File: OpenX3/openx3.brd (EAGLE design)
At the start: 46.7 x 49.1 mm, 34 parts, among them IC1 24AA256SN, J1 BM20B-SRDS-G-TF(LF)(SN), J2 SM12B-SRSS-TB(LF)(SN), J3 53398-0271, J4 1734260-3, U1 LC4256V-75TN100CTQFP100-L, U2 AM29F016D-70EF, U3 AM29F002BB90EI

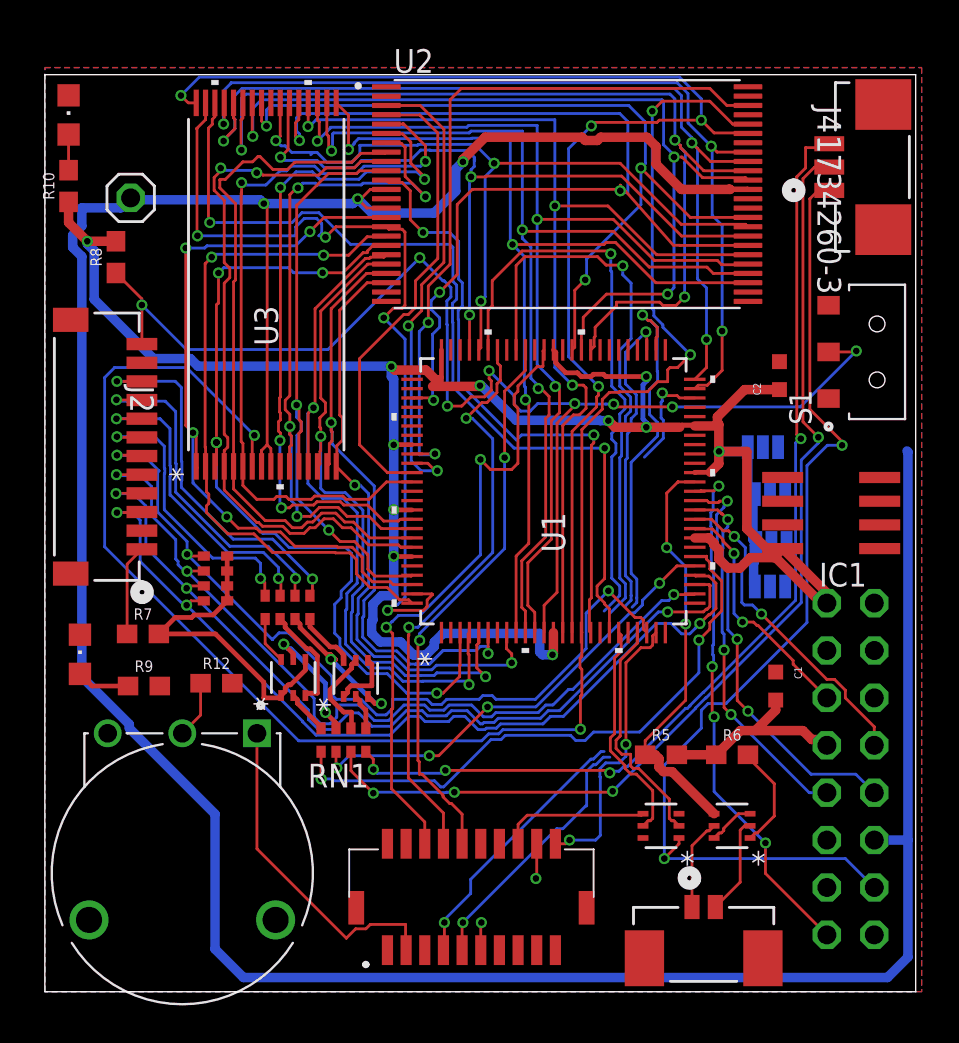
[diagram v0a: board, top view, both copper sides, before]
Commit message: routing complete... passes DRC
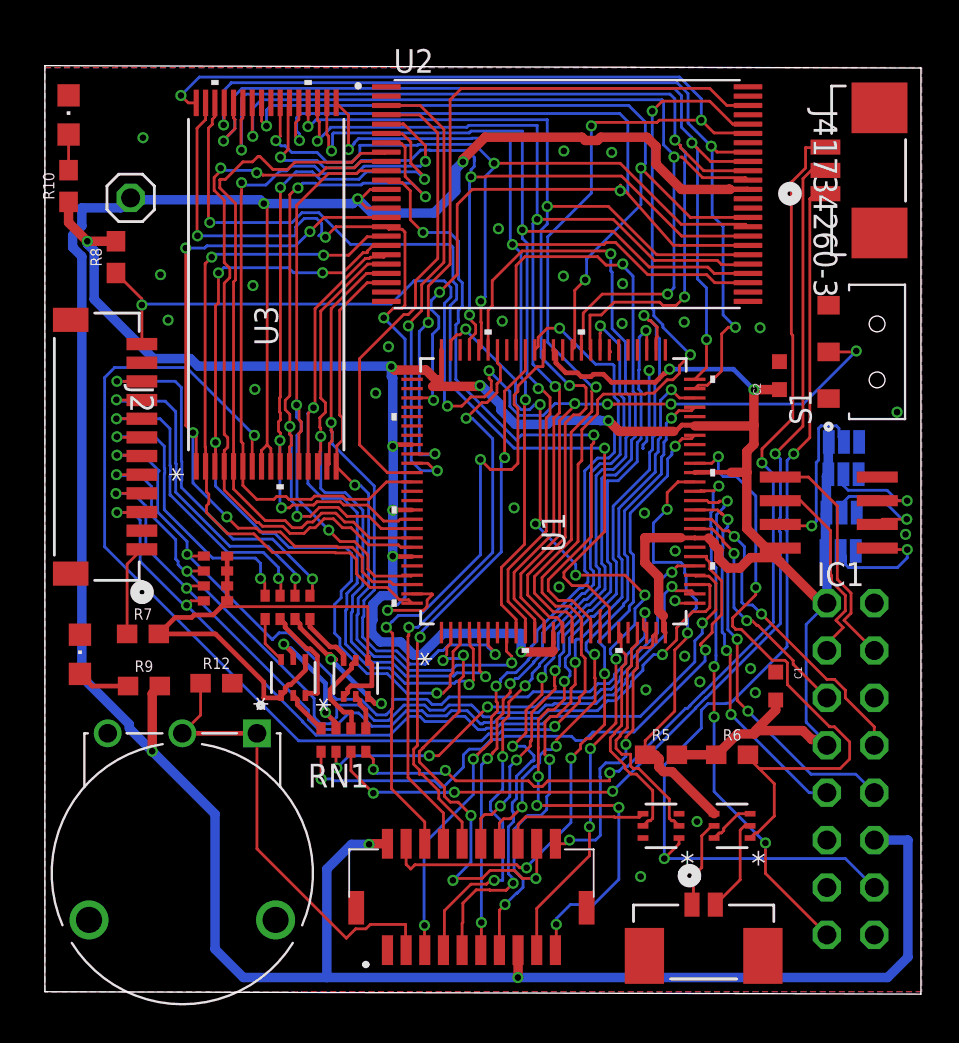
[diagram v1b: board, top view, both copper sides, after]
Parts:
- moved JPWP 4.35 mm to (41.6, 28.2)
- moved JPA0 4.24 mm to (41.4, 22.4)
- moved JPA1 4.10 mm to (41.4, 24.4)
- moved JPA2 4.08 mm to (41.5, 26.5)
- moved J4 0.27 mm to (40.6, 42.7)
- moved IC1 0.13 mm to (40.7, 24.4)
- moved J3 0.13 mm to (34.0, 1.40)
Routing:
- net TDO: track 0.00 -> 44.2 mm, vias 0 -> 8
- net RW: track 0.00 -> 42.5 mm, vias 0 -> 4
- net DB4: track 1.49 -> 39.1 mm, vias 1 -> 4
- net RS: track 0.00 -> 35.6 mm, vias 0 -> 4
- net DB6: track 5.79 -> 36.8 mm, vias 1 -> 4
- net DB7: track 0.00 -> 29.3 mm, vias 0 -> 4
- net N$61: track 5.65 -> 33.4 mm, vias 0 -> 2
- net TMS: track 19.5 -> 46.4 mm, vias 1 -> 6
- net TDI: track 1.88 -> 24.4 mm, vias 1 -> 5
- net +3V3: track 136.6 -> 153.1 mm, vias 11 -> 10
- net DB5: track 16.9 -> 33.1 mm, vias 1 -> 4
- net SDA: track 0.00 -> 12.6 mm
- net SCL: track 0.00 -> 10.8 mm
- net N$4: track 21.2 -> 31.9 mm
- net DB2: track 44.8 -> 54.8 mm, vias 2 -> 4
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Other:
- board size 46.7 x 49.1 mm -> 46.9 x 49.8 mm
